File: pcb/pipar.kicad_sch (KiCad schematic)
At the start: 62 parts, among them SW1 SW_Wuerth_450301014042, SW2 SW_Wuerth_450301014042, U1 Seeeduino Xiao nRF52840, U2 nice_nano

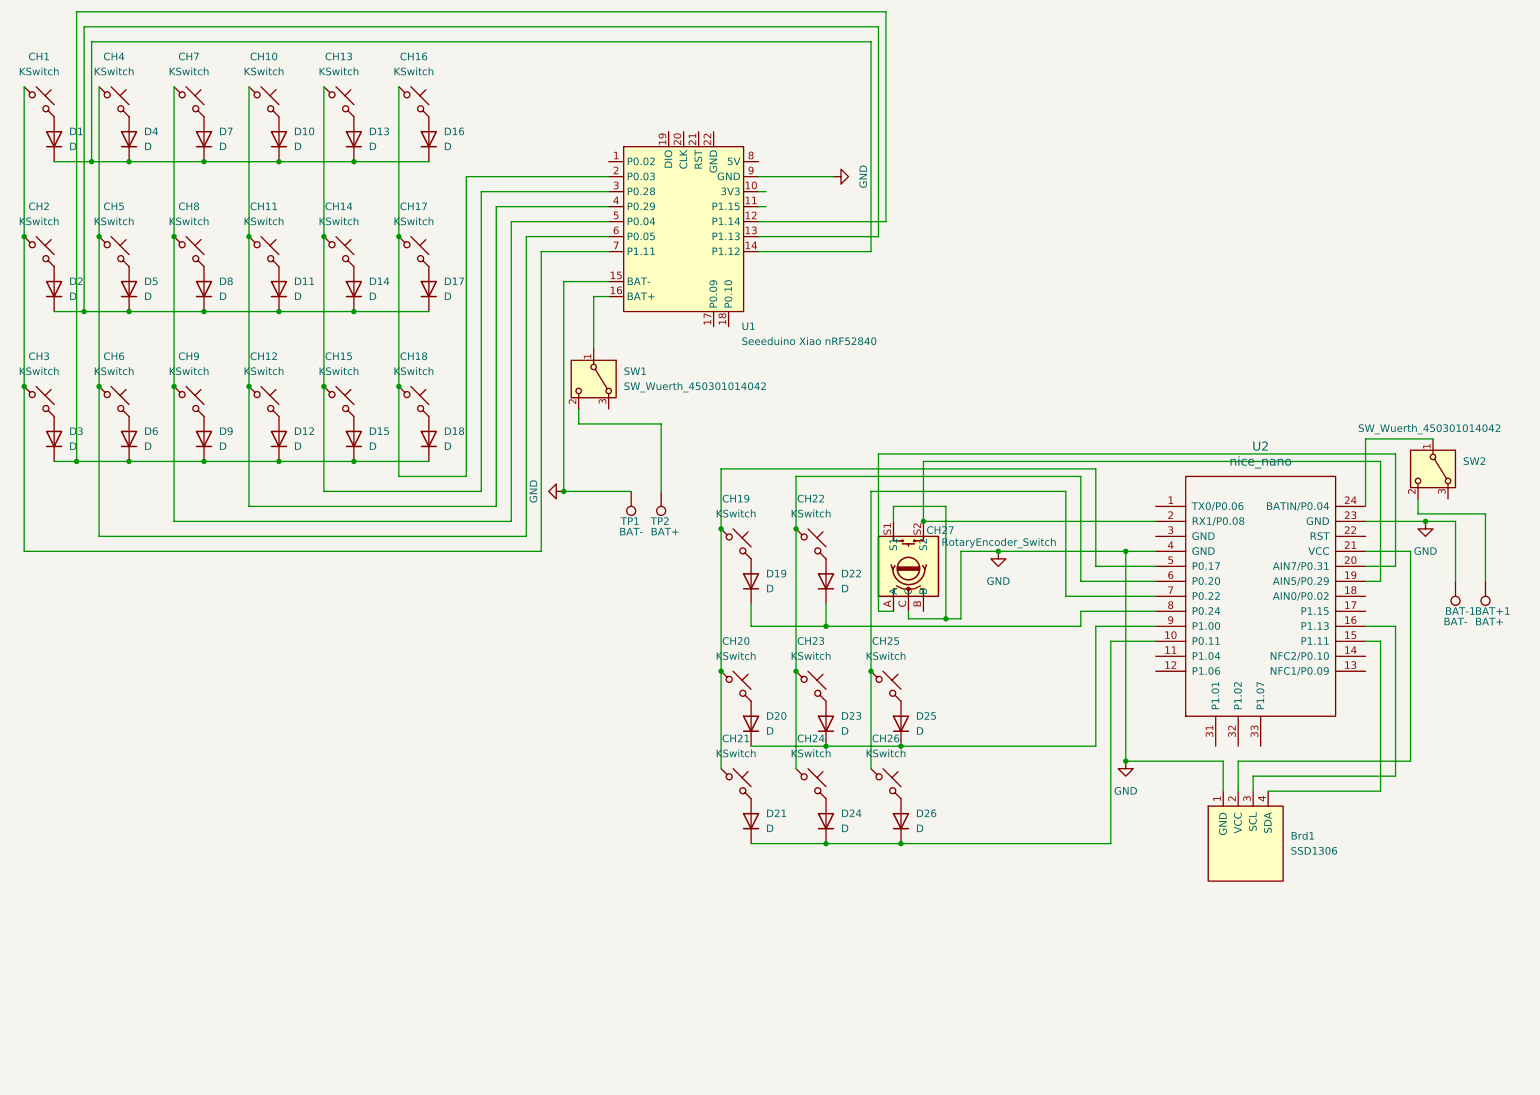
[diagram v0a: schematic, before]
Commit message: Improved schematics and PCBs
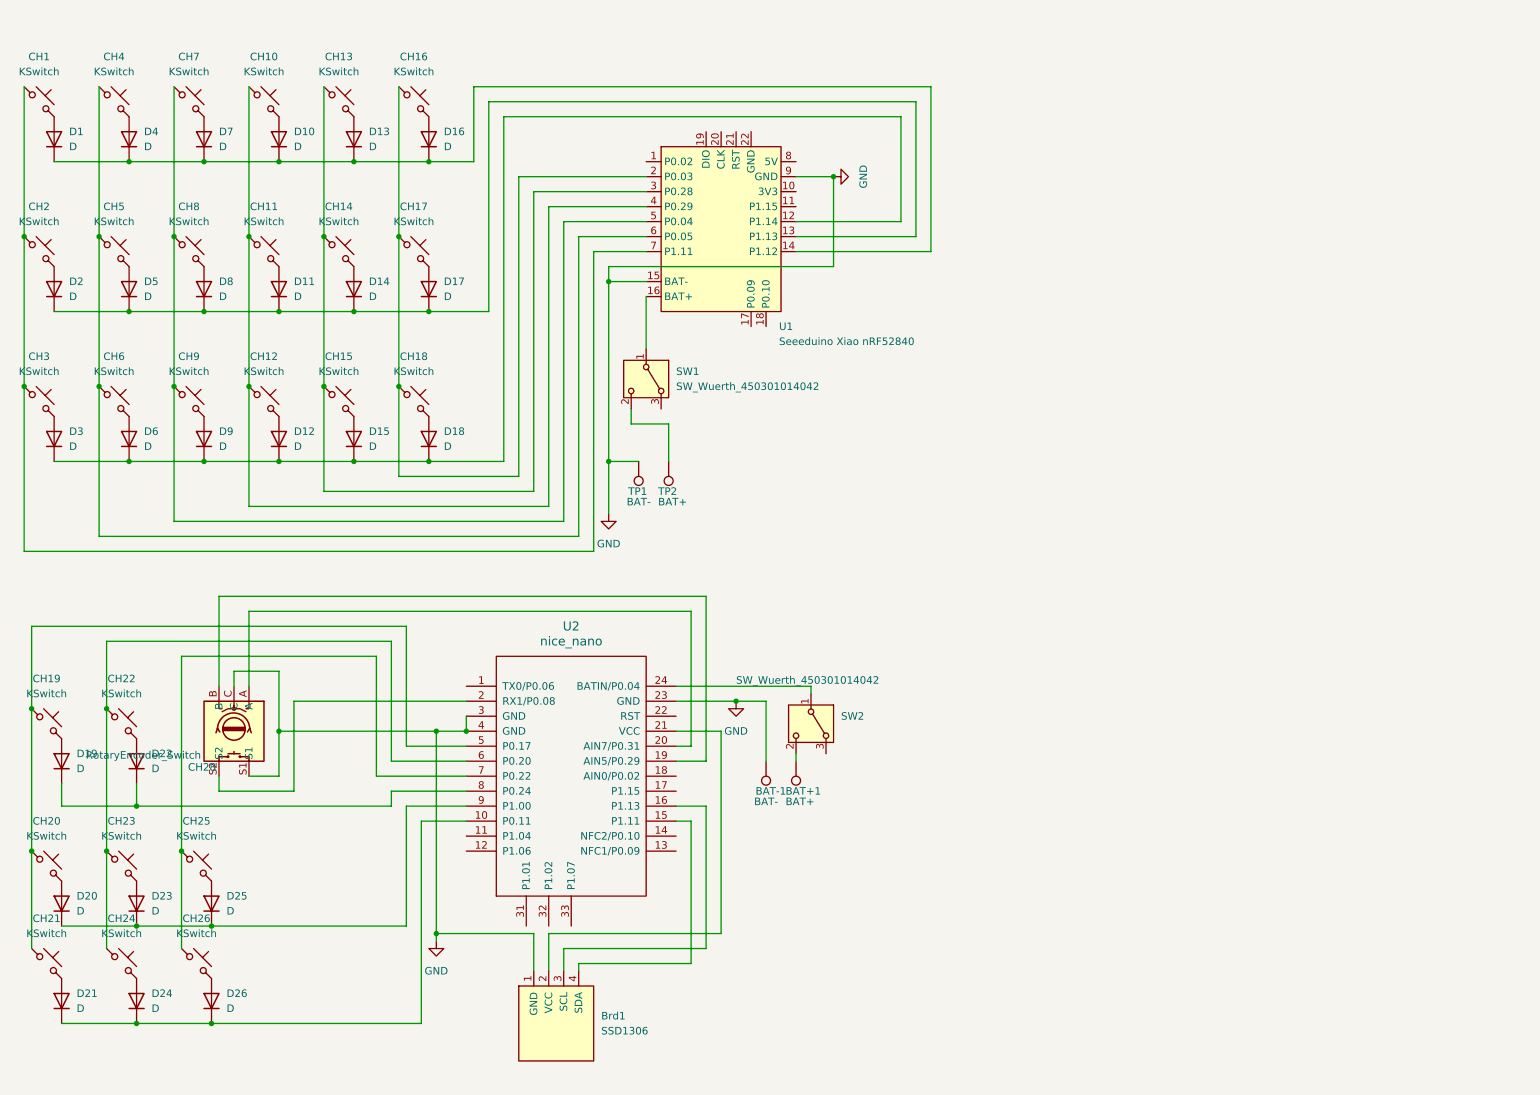
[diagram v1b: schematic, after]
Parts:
- removed CH27: RotaryEncoder_Switch, Rotary_Encoder:RotaryEncoder_Bourns_Vertical_PEL11L-4xxxF-Sxxxx_1, symbol Device:RotaryEncoder_Switch
- added CH28: RotaryEncoder_Switch, Rotary_Encoder:RotaryEncoder_Bourns_Vertical_PEL11L-4xxxF-Sxxxx_1, symbol Device:RotaryEncoder_Switch
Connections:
- net GND: now also U2.3 (GND), CH28.C, CH28.S1
- net at U2.19 (AIN5/P0.29): now also CH28.B; no longer U2.2 (RX1/P0.08)
- net at U2.20 (AIN7/P0.31): now also CH28.A
- new net: CH28.S2, U2.2 (RX1/P0.08)
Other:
- moved on the sheet: BAT+1, BAT-1, Brd1, CH19, CH20, CH21, CH22, CH23, CH24, CH25, CH26, D19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

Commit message: updates pcb and zmk, forgot to use i2c pins
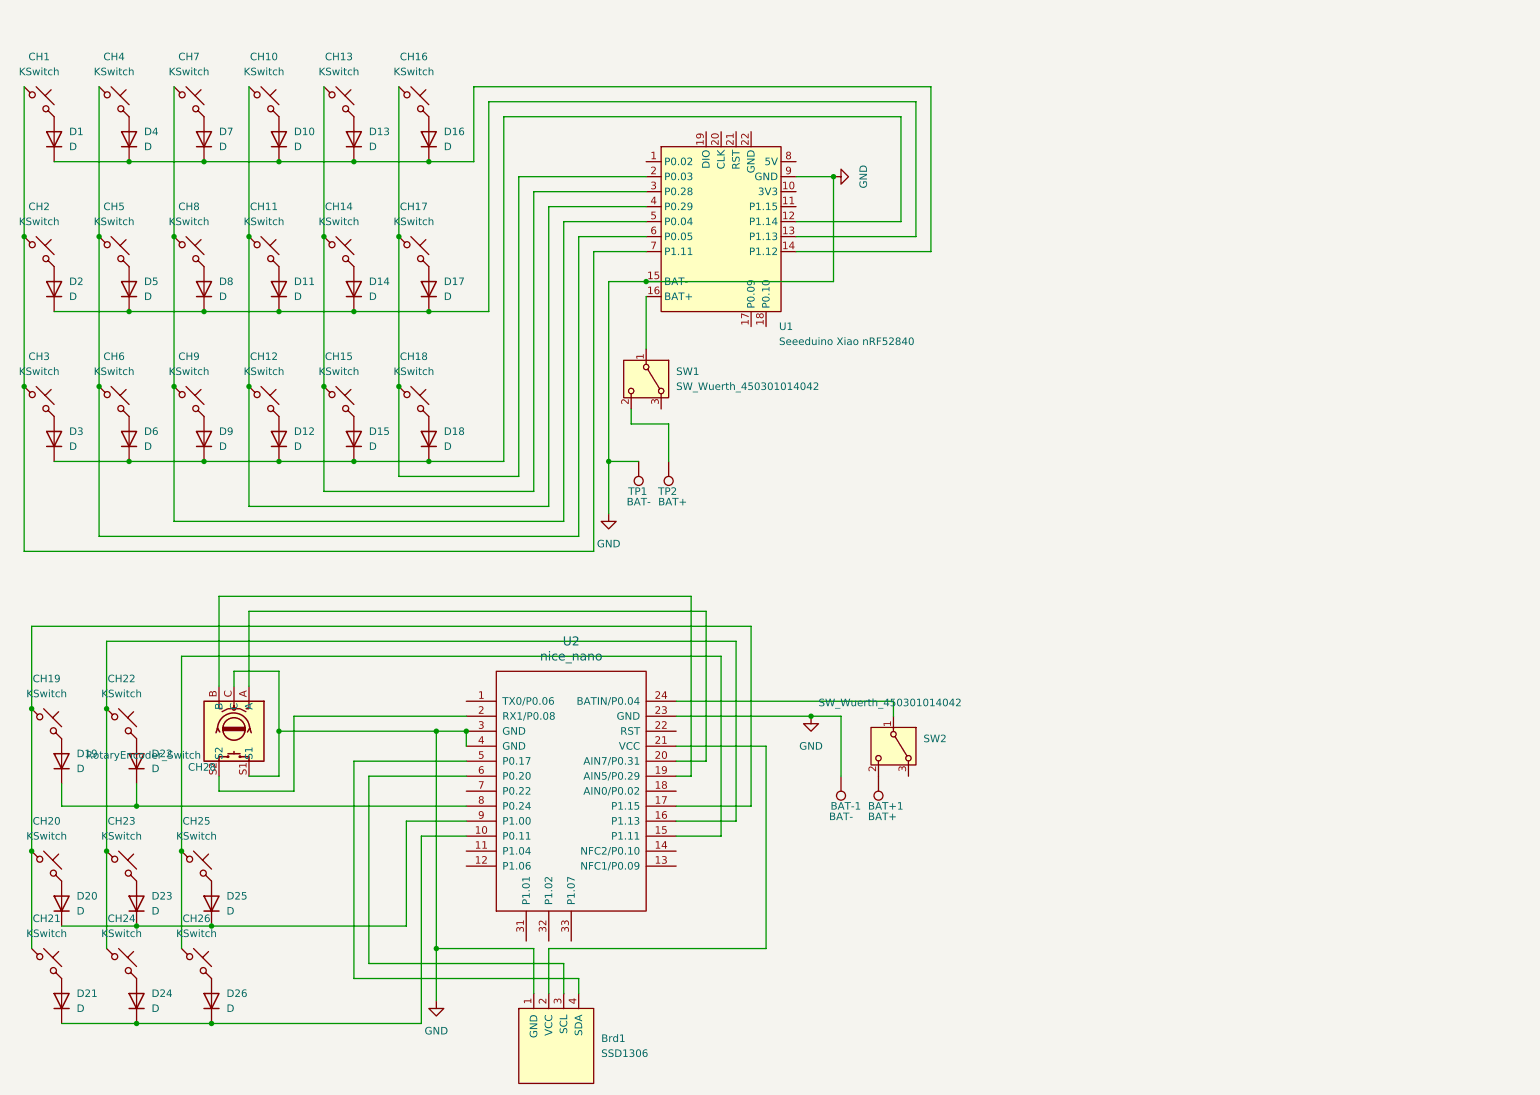
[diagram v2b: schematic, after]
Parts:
- BAT+1, BAT-1, Brd1, CH1, CH10, CH11, CH12, CH13, CH14, CH15, CH16, CH17, CH18, CH19, CH2, CH20, CH21, CH22, CH23, CH24, CH25, CH26, CH3, CH4, CH5, CH6, CH7, CH8, CH9, TP1, TP2, U2: now left out of the parts list
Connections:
- net at CH22.1, CH23.1, CH24.1: now also U2.16 (P1.13); no longer U2.6 (P0.20)
- net at Brd1.3 (SCL): now also U2.6 (P0.20); no longer U2.16 (P1.13)
- net at Brd1.4 (SDA): now also U2.5 (P0.17); no longer U2.15 (P1.11)
- net at U2.17 (P1.15): now also CH19.1, CH20.1, CH21.1
- net at CH25.1, CH26.1: now also U2.15 (P1.11); no longer U2.7 (P0.22)
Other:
- moved on the sheet: BAT+1, BAT-1, Brd1, SW2, U2
